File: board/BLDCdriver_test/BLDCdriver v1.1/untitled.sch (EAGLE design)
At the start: 28 parts, among them M1 JST-XH-03-PIN-LONG-PAD, X1 JST-XH-02-PIN-LONG-PAD, X2 JST-XH-06-PIN-ROUND-PAD, X4 JST-XH-04-PIN-ROUND-PAD

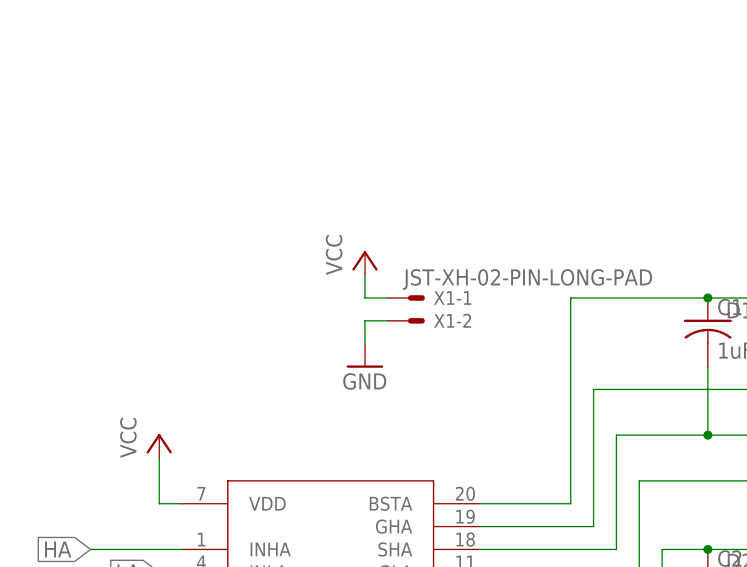
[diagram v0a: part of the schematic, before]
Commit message: update motordriver
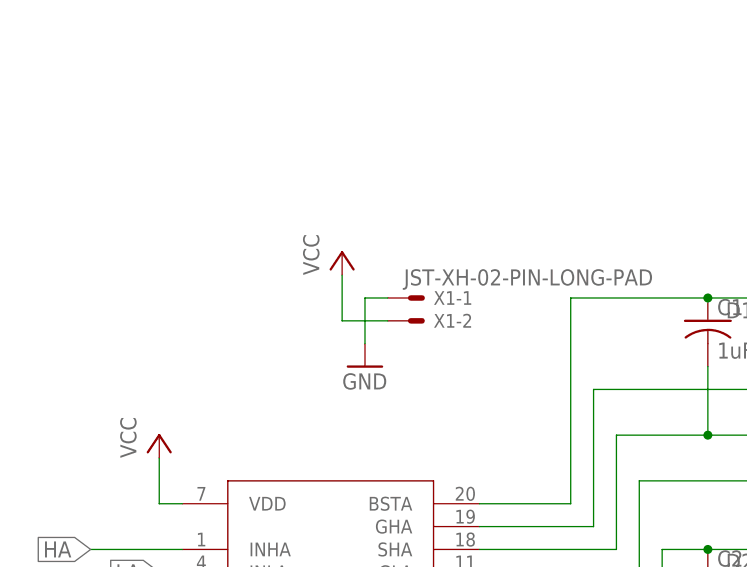
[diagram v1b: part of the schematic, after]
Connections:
- net GND: now also X1-1.S; no longer X1-2.S
- net VCC: now also X1-2.S; no longer X1-1.S
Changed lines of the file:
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@@
 <attribute name="VALUE" x="24.638" y="95.377" size="1.778" layer="96"/>
 </instance>
-<instance part="P+5" gate="VCC" x="20.32" y="99.06" smashed="yes">
-<attribute name="VALUE" x="17.78" y="96.52" size="1.778" layer="96" rot="R90"/>
+<instance part="P+5" gate="VCC" x="17.78" y="99.06" smashed="yes">
+<attribute name="VALUE" x="15.24" y="96.52" size="1.778" layer="96" rot="R90"/>
 </instance>
 <instance part="GND3" gate="1" x="20.32" y="86.36" smashed="yes">
@@
 </segment>
 <segment>
-<pinref part="X1" gate="-2" pin="S"/>
-<wire x1="22.86" y1="91.44" x2="20.32" y2="91.44" width="0.1524" layer="91"/>
-<wire x1="20.32" y1="91.44" x2="20.32" y2="88.9" width="0.1524" layer="91"/>
 <pinref part="GND3" gate="1" pin="GND"/>
+<pinref part="X1" gate="-1" pin="S"/>
+<wire x1="20.32" y1="88.9" x2="20.32" y2="93.98" width="0.1524" layer="91"/>
+<wire x1="20.32" y1="93.98" x2="22.86" y2="93.98" width="0.1524" layer="91"/>
 </segment>
 <segment>
@@
 </segment>
 <segment>
-<pinref part="X1" gate="-1" pin="S"/>
-<wire x1="22.86" y1="93.98" x2="20.32" y2="93.98" width="0.1524" layer="91"/>
-<wire x1="20.32" y1="93.98" x2="20.32" y2="96.52" width="0.1524" layer="91"/>
 <pinref part="P+5" gate="VCC" pin="VCC"/>
-</segment>
-</net>
+<pinref part="X1" gate="-2" pin="S"/>
+<wire x1="17.78" y1="96.52" x2="17.78" y2="91.44" width="0.1524" layer="91"/>
+<wire x1="17.78" y1="91.44" x2="22.86" y2="91.44" width="0.1524" layer="91"/>
+</segment>
+</net>

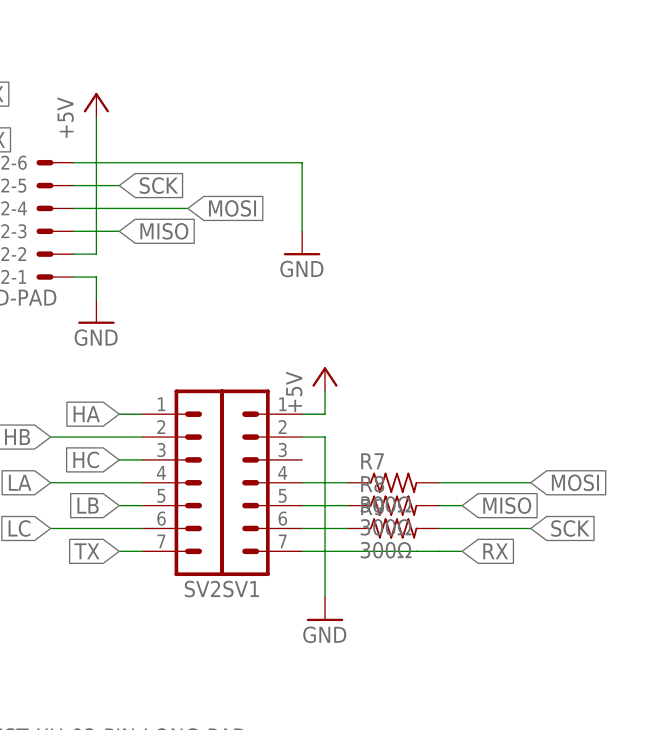
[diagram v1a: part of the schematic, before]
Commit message: marge前のファイル
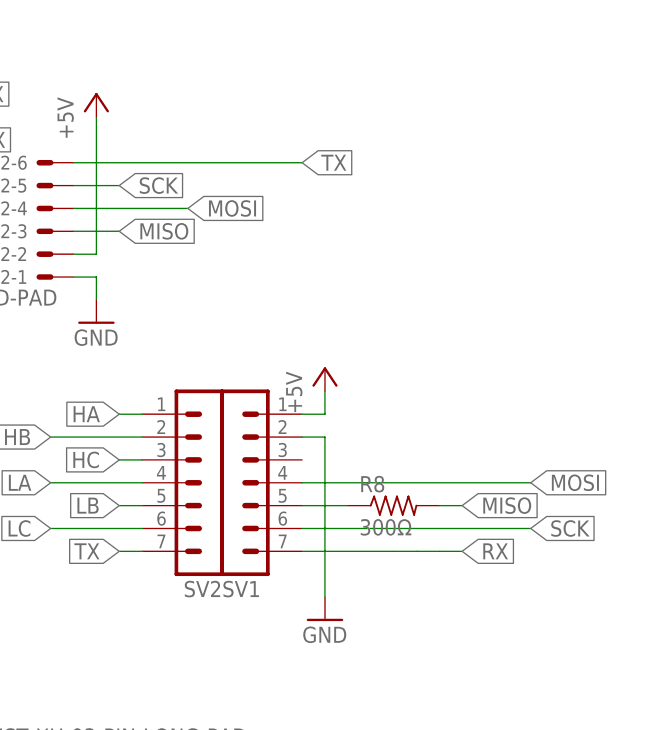
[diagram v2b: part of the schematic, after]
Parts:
- removed R7, R9: 300Ω, adafruit:R-US_M2012
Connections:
- removed net N$11: R7.1, SV1.4
- removed net N$20: R9.1, SV1.6
- net GND: no longer X2-6.S
- net MOSI: now also SV1.4; no longer R7.2
- net SCK: now also SV1.6; no longer R9.2
- net TX: now also X2-6.S
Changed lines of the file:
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@@
 <?xml version="1.0" encoding="utf-8"?>
 <!DOCTYPE eagle SYSTEM "eagle.dtd">
-<eagle version="9.6.1">
+<eagle version="9.6.2">
 <drawing>
 <settings>
@@
 <part name="P+8" library="supply1" library_urn="urn:adsk.eagle:library:371" deviceset="+5V" device=""/>
 <part name="GND6" library="supply1" library_urn="urn:adsk.eagle:library:371" deviceset="GND" device=""/>
-<part name="R7" library="adafruit" deviceset="R-US_" device="M2012" value="300Ω"/>
 <part name="R8" library="adafruit" deviceset="R-US_" device="M2012" value="300Ω"/>
-<part name="R9" library="adafruit" deviceset="R-US_" device="M2012" value="300Ω"/>
-<part name="GND7" library="supply1" library_urn="urn:adsk.eagle:library:371" deviceset="GND" device=""/>
 </parts>
 <sheets>
@@
 <attribute name="VALUE" x="83.82" y="116.84" size="1.778" layer="96"/>
 </instance>
-<instance part="R7" gate="G$1" x="137.16" y="86.36" smashed="yes">
-<attribute name="NAME" x="133.35" y="87.8586" size="1.778" layer="95"/>
-<attribute name="VALUE" x="133.35" y="83.058" size="1.778" layer="96"/>
-</instance>
 <instance part="R8" gate="G$1" x="137.16" y="83.82" smashed="yes">
 <attribute name="NAME" x="133.35" y="85.3186" size="1.778" layer="95"/>
 <attribute name="VALUE" x="133.35" y="80.518" size="1.778" layer="96"/>
-</instance>
-<instance part="R9" gate="G$1" x="137.16" y="81.28" smashed="yes">
-<attribute name="NAME" x="133.35" y="82.7786" size="1.778" layer="95"/>
-<attribute name="VALUE" x="133.35" y="77.978" size="1.778" layer="96"/>
-</instance>
-<instance part="GND7" gate="1" x="127" y="111.76" smashed="yes">
-<attribute name="VALUE" x="124.46" y="109.22" size="1.778" layer="96"/>
 </instance>
 </instances>
@@
 <pinref part="GND6" gate="1" pin="GND"/>
 </segment>
-<segment>
-<pinref part="X2" gate="-6" pin="S"/>
-<wire x1="101.6" y1="121.92" x2="127" y2="121.92" width="0.1524" layer="91"/>
-<wire x1="127" y1="121.92" x2="127" y2="114.3" width="0.1524" layer="91"/>
-<pinref part="GND7" gate="1" pin="GND"/>
-</segment>
 </net>
 <net name="N$12" class="0">
@@
 <segment>
 <label x="152.4" y="86.36" size="1.778" layer="95" xref="yes"/>
-<pinref part="R7" gate="G$1" pin="2"/>
-<wire x1="142.24" y1="86.36" x2="152.4" y2="86.36" width="0.1524" layer="91"/>
+<pinref part="SV1" gate="1" pin="4"/>
+<wire x1="127" y1="86.36" x2="152.4" y2="86.36" width="0.1524" layer="91"/>
 </segment>
 </net>
@@
 <segment>
 <label x="152.4" y="81.28" size="1.778" layer="95" xref="yes"/>
-<pinref part="R9" gate="G$1" pin="2"/>
-<wire x1="142.24" y1="81.28" x2="152.4" y2="81.28" width="0.1524" layer="91"/>
+<pinref part="SV1" gate="1" pin="6"/>
+<wire x1="127" y1="81.28" x2="152.4" y2="81.28" width="0.1524" layer="91"/>
 </segment>
 </net>
@@
 <label x="88.9" y="129.54" size="1.778" layer="95" xref="yes"/>
 </segment>
+<segment>
+<pinref part="X2" gate="-6" pin="S"/>
+<wire x1="101.6" y1="121.92" x2="127" y2="121.92" width="0.1524" layer="91"/>
+<label x="127" y="121.92" size="1.778" layer="95" xref="yes"/>
+</segment>
 </net>
 <net name="LC" class="0">
@@
 </segment>
 </net>
-<net name="N$11" class="0">
-<segment>
-<pinref part="SV1" gate="1" pin="4"/>
-<wire x1="132.08" y1="86.36" x2="127" y2="86.36" width="0.1524" layer="91"/>
-<pinref part="R7" gate="G$1" pin="1"/>
-</segment>
-</net>
-<net name="N$20" class="0">
-<segment>
-<pinref part="SV1" gate="1" pin="6"/>
-<wire x1="127" y1="81.28" x2="132.08" y2="81.28" width="0.1524" layer="91"/>
-<pinref part="R9" gate="G$1" pin="1"/>
-</segment>
-</net>

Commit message: Revert "Merge remote-tracking branch 'origin/Develop' into feature_#37"
This reverts commit cb103155361e8766478c6830db153463370c0739, reversing
changes made to 84e093fe944e1f8653a6822ff34e6f8740617cb5.
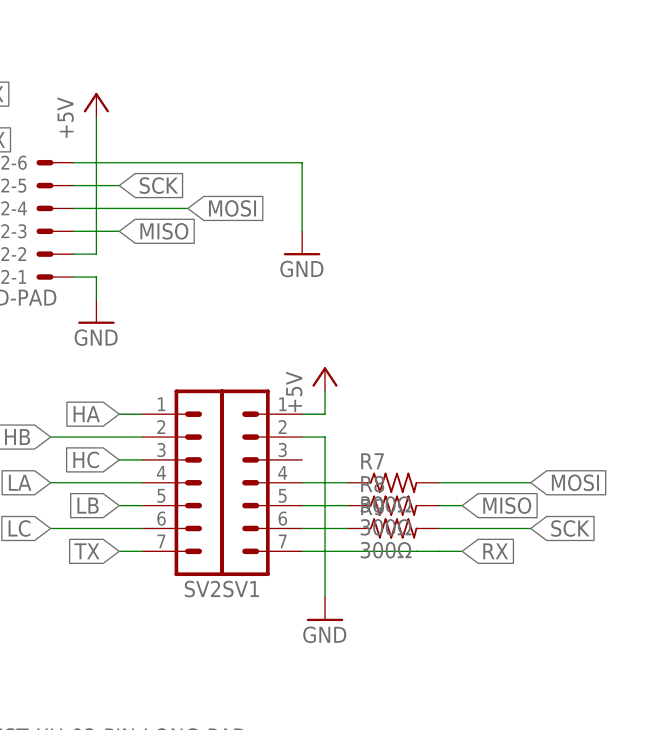
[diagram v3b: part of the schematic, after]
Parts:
- added R7, R9: 300Ω, adafruit:R-US_M2012
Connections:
- new net N$11: R7.1, SV1.4
- new net N$20: R9.1, SV1.6
- net GND: now also X2-6.S
- net MOSI: now also R7.2; no longer SV1.4
- net SCK: now also R9.2; no longer SV1.6
- net TX: no longer X2-6.S
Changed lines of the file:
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@@
 <?xml version="1.0" encoding="utf-8"?>
 <!DOCTYPE eagle SYSTEM "eagle.dtd">
-<eagle version="9.6.2">
+<eagle version="9.6.1">
 <drawing>
 <settings>
@@
 <part name="P+8" library="supply1" library_urn="urn:adsk.eagle:library:371" deviceset="+5V" device=""/>
 <part name="GND6" library="supply1" library_urn="urn:adsk.eagle:library:371" deviceset="GND" device=""/>
+<part name="R7" library="adafruit" deviceset="R-US_" device="M2012" value="300Ω"/>
 <part name="R8" library="adafruit" deviceset="R-US_" device="M2012" value="300Ω"/>
+<part name="R9" library="adafruit" deviceset="R-US_" device="M2012" value="300Ω"/>
+<part name="GND7" library="supply1" library_urn="urn:adsk.eagle:library:371" deviceset="GND" device=""/>
 </parts>
 <sheets>
@@
 <attribute name="VALUE" x="83.82" y="116.84" size="1.778" layer="96"/>
 </instance>
+<instance part="R7" gate="G$1" x="137.16" y="86.36" smashed="yes">
+<attribute name="NAME" x="133.35" y="87.8586" size="1.778" layer="95"/>
+<attribute name="VALUE" x="133.35" y="83.058" size="1.778" layer="96"/>
+</instance>
 <instance part="R8" gate="G$1" x="137.16" y="83.82" smashed="yes">
 <attribute name="NAME" x="133.35" y="85.3186" size="1.778" layer="95"/>
 <attribute name="VALUE" x="133.35" y="80.518" size="1.778" layer="96"/>
+</instance>
+<instance part="R9" gate="G$1" x="137.16" y="81.28" smashed="yes">
+<attribute name="NAME" x="133.35" y="82.7786" size="1.778" layer="95"/>
+<attribute name="VALUE" x="133.35" y="77.978" size="1.778" layer="96"/>
+</instance>
+<instance part="GND7" gate="1" x="127" y="111.76" smashed="yes">
+<attribute name="VALUE" x="124.46" y="109.22" size="1.778" layer="96"/>
 </instance>
 </instances>
@@
 <pinref part="GND6" gate="1" pin="GND"/>
 </segment>
+<segment>
+<pinref part="X2" gate="-6" pin="S"/>
+<wire x1="101.6" y1="121.92" x2="127" y2="121.92" width="0.1524" layer="91"/>
+<wire x1="127" y1="121.92" x2="127" y2="114.3" width="0.1524" layer="91"/>
+<pinref part="GND7" gate="1" pin="GND"/>
+</segment>
 </net>
 <net name="N$12" class="0">
@@
 <segment>
 <label x="152.4" y="86.36" size="1.778" layer="95" xref="yes"/>
-<pinref part="SV1" gate="1" pin="4"/>
-<wire x1="127" y1="86.36" x2="152.4" y2="86.36" width="0.1524" layer="91"/>
+<pinref part="R7" gate="G$1" pin="2"/>
+<wire x1="142.24" y1="86.36" x2="152.4" y2="86.36" width="0.1524" layer="91"/>
 </segment>
 </net>
@@
 <segment>
 <label x="152.4" y="81.28" size="1.778" layer="95" xref="yes"/>
-<pinref part="SV1" gate="1" pin="6"/>
-<wire x1="127" y1="81.28" x2="152.4" y2="81.28" width="0.1524" layer="91"/>
+<pinref part="R9" gate="G$1" pin="2"/>
+<wire x1="142.24" y1="81.28" x2="152.4" y2="81.28" width="0.1524" layer="91"/>
 </segment>
 </net>
@@
 <label x="88.9" y="129.54" size="1.778" layer="95" xref="yes"/>
 </segment>
-<segment>
-<pinref part="X2" gate="-6" pin="S"/>
-<wire x1="101.6" y1="121.92" x2="127" y2="121.92" width="0.1524" layer="91"/>
-<label x="127" y="121.92" size="1.778" layer="95" xref="yes"/>
-</segment>
 </net>
 <net name="LC" class="0">
@@
 </segment>
 </net>
+<net name="N$11" class="0">
+<segment>
+<pinref part="SV1" gate="1" pin="4"/>
+<wire x1="132.08" y1="86.36" x2="127" y2="86.36" width="0.1524" layer="91"/>
+<pinref part="R7" gate="G$1" pin="1"/>
+</segment>
+</net>
+<net name="N$20" class="0">
+<segment>
+<pinref part="SV1" gate="1" pin="6"/>
+<wire x1="127" y1="81.28" x2="132.08" y2="81.28" width="0.1524" layer="91"/>
+<pinref part="R9" gate="G$1" pin="1"/>
+</segment>
+</net>
